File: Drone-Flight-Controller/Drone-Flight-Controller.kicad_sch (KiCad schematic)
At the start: 58 parts, among them J1 Screw_Terminal_01x02, J10 Conn_ARM_SWD_TagConnect_TC203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, J2 USB_B_Micro, J3 Screw_Terminal_01x03, J4 Screw_Terminal_01x03, J5 Screw_Terminal_01x03, J6 Screw_Terminal_01x03, J7 Screw_Terminal_01x02, J8 Screw_Terminal_01x03, SW1 SW_SPDT, U1 LMR51430, U2 NCP1117-3.3_SOT223, U3 STM32F401CBUx, U4 USBLC6-2SC6, U5 ADC101C021CIMK, U6 MPU-6050, U7 BMP280, Y1 16MHz

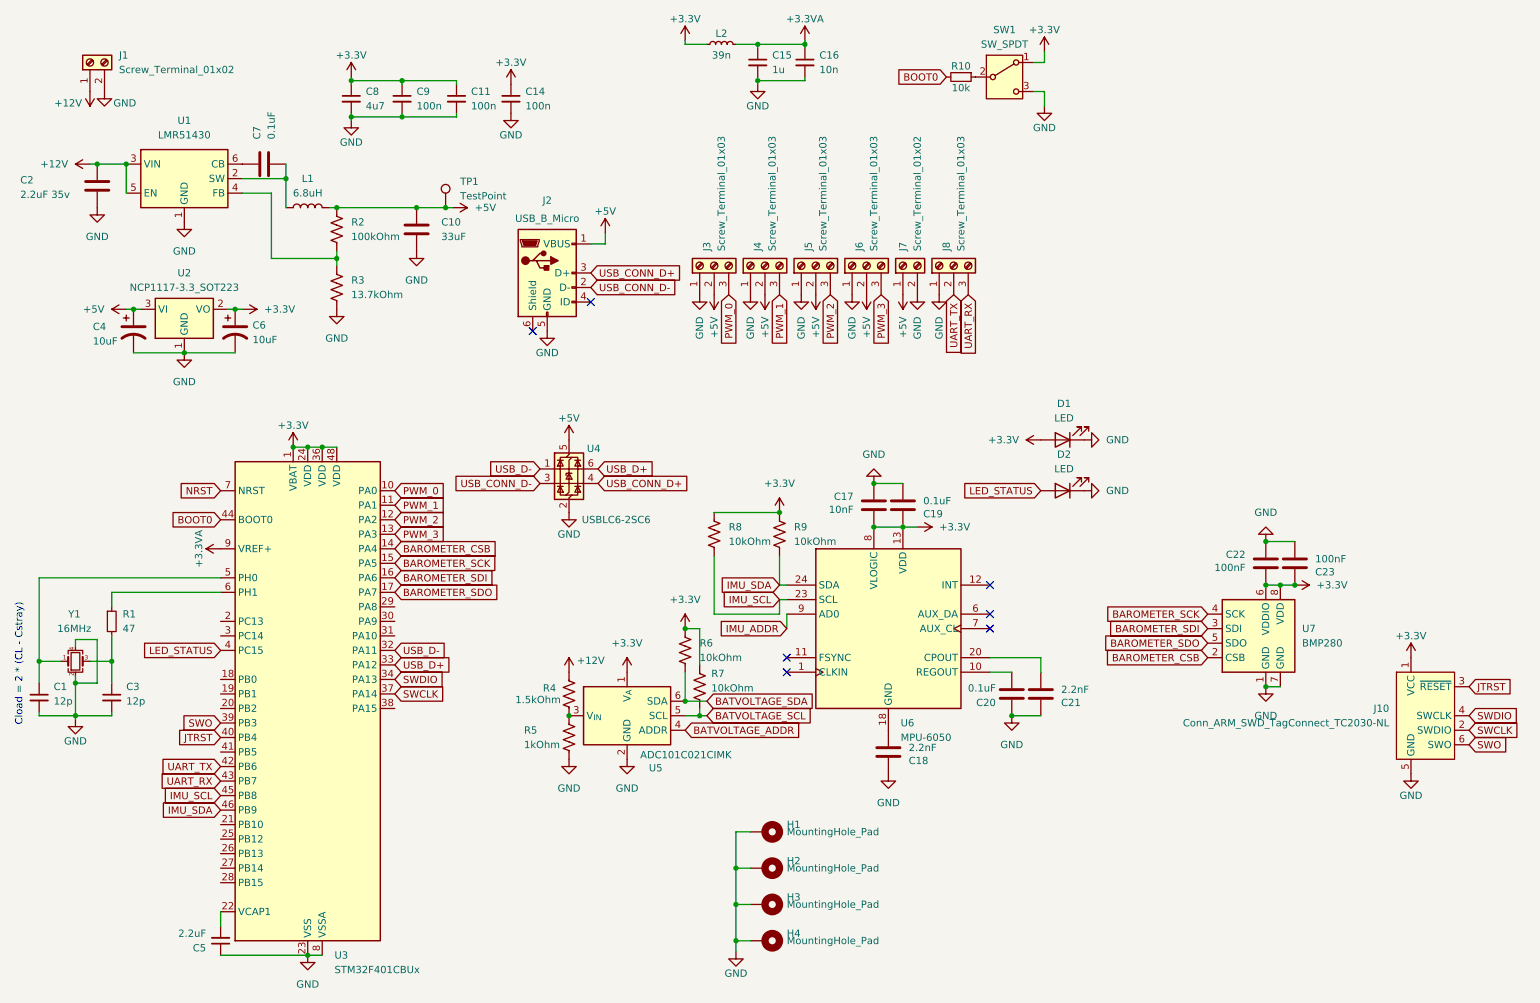
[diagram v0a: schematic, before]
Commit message: forgot to save
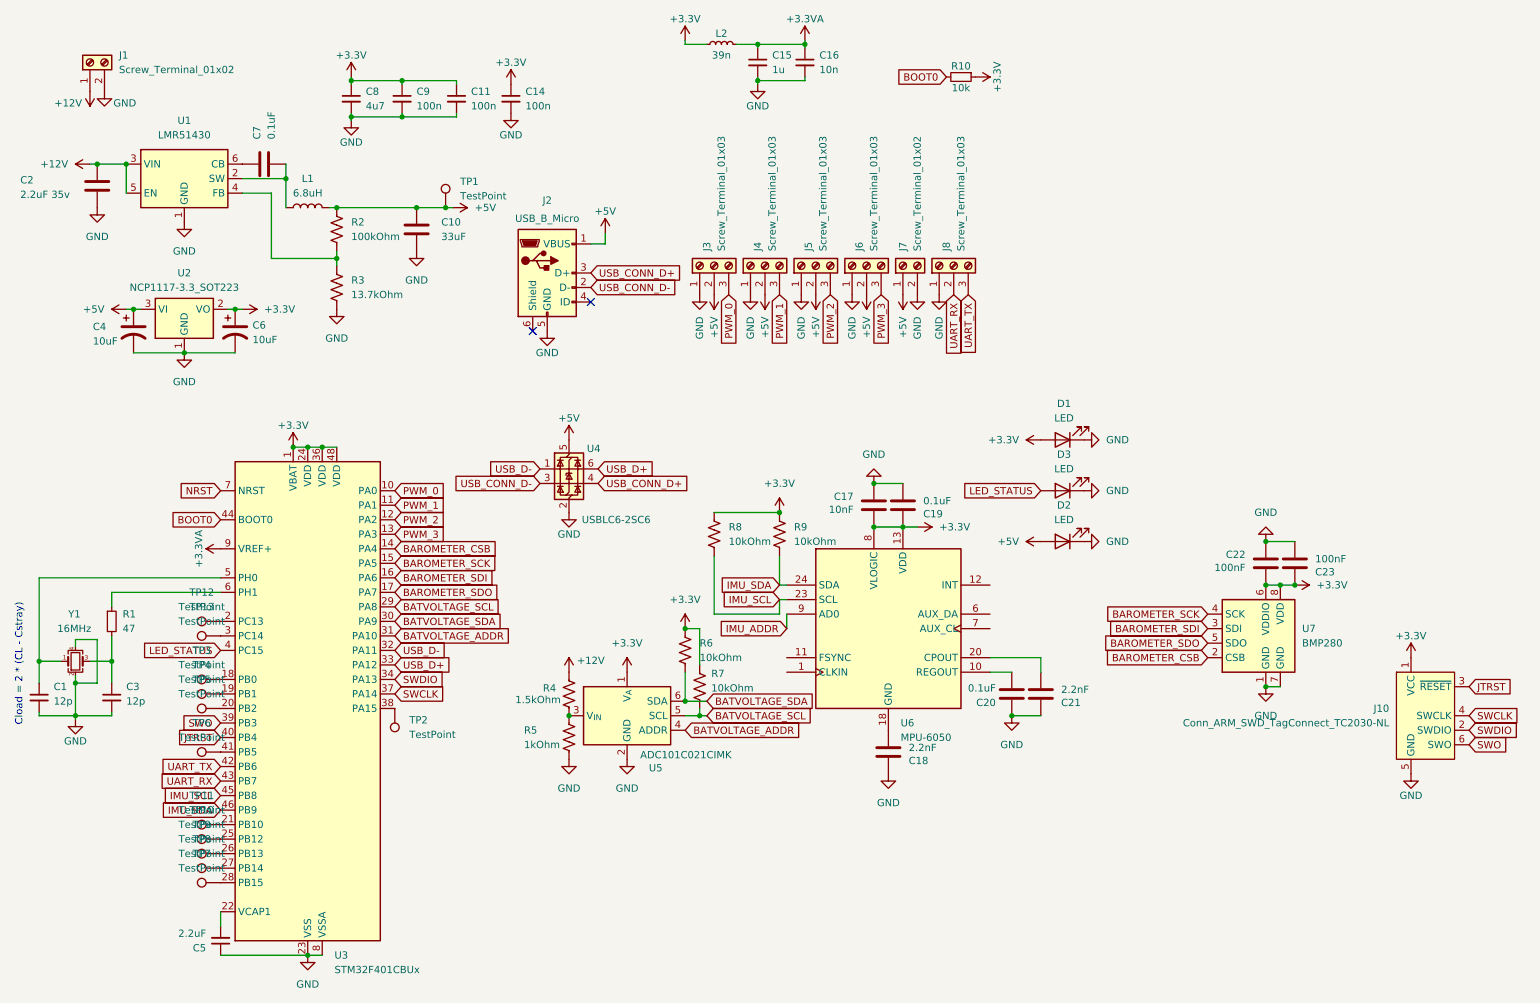
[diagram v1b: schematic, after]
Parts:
- removed H1, H2, H3, H4: MountingHole_Pad, MountingHole:MountingHole_4.3mm_M4_Pad_Via, symbol Mechanical:MountingHole_Pad
- removed SW1: SW_SPDT, Button_Switch_SMD:SW_SPDT_PCM12, symbol Switch:SW_SPDT
- added D2: LED, LED_SMD:LED_0402_1005Metric, symbol Device:LED
- added TP10, TP11, TP12, TP13, TP2, TP3, TP4, TP5, TP6, TP7, TP8, TP9: TestPoint, TestPoint:TestPoint_Pad_D1.0mm, symbol Connector:TestPoint
- C10: footprint Capacitor_THT:C_Radial_D4.0mm_H5.0mm_P1.50mm -> Capacitor_SMD:C_0504_1310Metric
- C2, C22, C23, C7: footprint Capacitor_THT:C_Radial_D4.0mm_H5.0mm_P1.50mm -> Capacitor_SMD:C_0402_1005Metric
- D1: footprint LED_THT:LED_D3.0mm -> LED_SMD:LED_0402_1005Metric
- D3: renamed from D2; footprint LED_THT:LED_D3.0mm -> LED_SMD:LED_0402_1005Metric
- R2, R3, R4, R5, R6, R7: footprint Resistor_THT:R_Axial_DIN0204_L3.6mm_D1.6mm_P7.62mm_Horizontal -> Resistor_SMD:R_0402_1005Metric
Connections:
- net +3.3V: now also R10.1
- net +5V: now also D2.2 (A)
- net BATVOLTAGE_ADDR: now also U3.31 (PA10)
- net BATVOLTAGE_SCL: now also U3.29 (PA8)
- net BATVOLTAGE_SDA: now also U3.30 (PA9)
- net GND: now also D2.1 (K)
- net SWCLK: now also J10.4 (SWCLK); no longer J10.2 (SWDIO)
- net SWDIO: now also J10.2 (SWDIO); no longer J10.4 (SWCLK)
- net UART_RX: now also J8.2 (Pin_2); no longer J8.3 (Pin_3)
- net UART_TX: now also J8.3 (Pin_3); no longer J8.2 (Pin_2)
- net at U3.18 (PB0): now also TP3.1
- net at U3.19 (PB1): now also TP4.1
- net at U3.2 (PC13): now also TP12.1
- net at U3.20 (PB2): now also TP5.1
- net at U3.21 (PB10): now also TP11.1
- net at U3.25 (PB12): now also TP10.1
- net at U3.26 (PB13): now also TP9.1
- net at U3.27 (PB14): now also TP8.1
- net at U3.28 (PB15): now also TP7.1
- net at U3.3 (PC14): now also TP13.1
- net at U3.38 (PA15): now also TP2.1
- net at U3.41 (PB5): now also TP6.1
- no-connect marks 7 -> 2
